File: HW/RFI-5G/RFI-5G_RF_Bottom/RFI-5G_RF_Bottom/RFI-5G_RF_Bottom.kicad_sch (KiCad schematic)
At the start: 42 parts, among them J1 Conn_01x03, J2 Conn_01x02, J3 Conn_01x03, J4 Conn_01x10, J5 SMP, J6 Conn_01x06_Female, U1 HMC8411, U2 SIM-14+, U3 LT5537, U4 LEE2-6+, U5 LEE2-6+, U7 HMC358

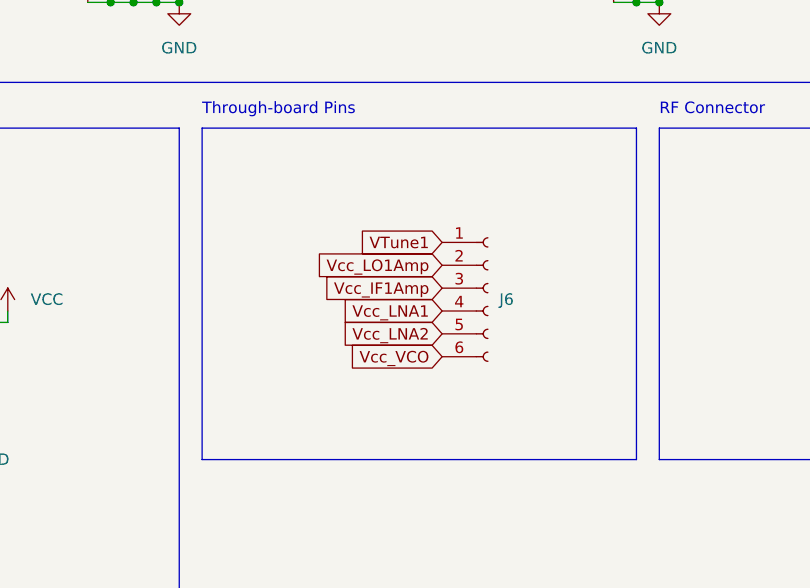
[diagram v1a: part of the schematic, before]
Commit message: PL boards
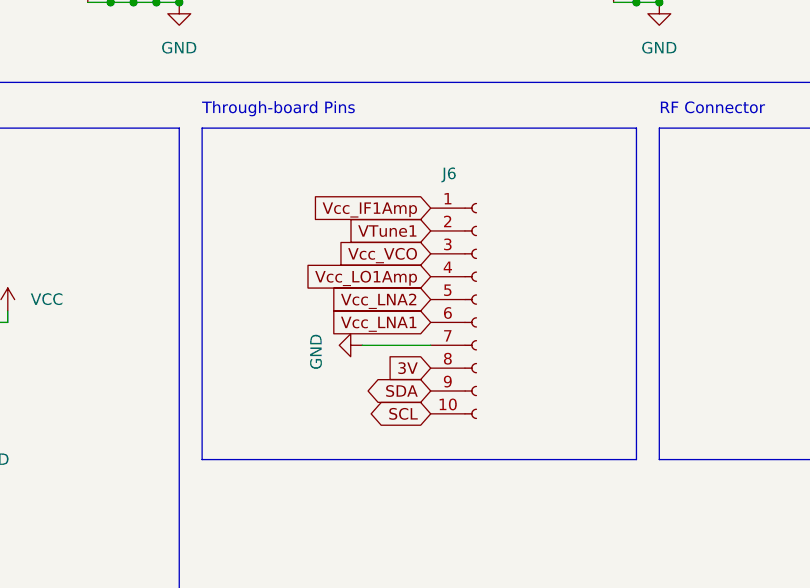
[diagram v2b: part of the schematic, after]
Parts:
- removed J6: Conn_01x06_Female, Connector_PinHeader_1.00mm:PinHeader_1x06_P1.00mm_Vertical, symbol Connector:Conn_01x06_Female
- added J6: Conn_01x10_Female, Connector_PinHeader_1.00mm:PinHeader_1x10_P1.00mm_Vertical, symbol Connector:Conn_01x10_Female
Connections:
- net 3V: now also J6.8 (Pin_8)
- net GND: now also J6.7 (Pin_7)
- net SCL: now also J6.10 (Pin_10)
- net SDA: now also J6.9 (Pin_9)
- net VTune1: now also J6.2 (Pin_2)
- net Vcc_IF1Amp: now also J6.1 (Pin_1)
- net Vcc_LNA1: now also J6.6 (Pin_6)
- net Vcc_LNA2: now also J6.5 (Pin_5)
- net Vcc_LO1Amp: now also J6.4 (Pin_4)
- net Vcc_VCO: now also J6.3 (Pin_3)
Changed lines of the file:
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@@
+    (stroke (width 0) (type default) (color 0 0 0 0))
+  )
+  (wire (pts (xy 104.14 148.59) (xy 111.76 148.59))
     (stroke (width 0) (type default) (color 0 0 0 0))
   )
@@
     (effects (font (size 1.27 1.27)) (justify left bottom))
   )
-  (global_label "Vcc_LO1Amp" (shape input) (at 113.03 139.7 180) (fields_autoplaced)
-    (effects (font (size 1.27 1.27)) (justify right))
-    (property "Intersheet References" "${INTERSHEET_REFS}" (id 0) (at 98.8845 139.6206 0)
+  (global_label "3V" (shape input) (at 111.76 151.13 180) (fields_autoplaced)
+    (effects (font (size 1.27 1.27)) (justify right))
+    (property "Intersheet References" "${INTERSHEET_REFS}" (id 0) (at 107.0488 151.0506 0)
       (effects (font (size 1.27 1.27)) (justify right) hide)
     )
@@
     )
   )
-  (global_label "Vcc_IF1Amp" (shape input) (at 113.03 142.24 180) (fields_autoplaced)
-    (effects (font (size 1.27 1.27)) (justify right))
-    (property "Intersheet References" "${INTERSHEET_REFS}" (id 0) (at 99.5498 142.1606 0)
-      (effects (font (size 1.27 1.27)) (justify right) hide)
-    )
-  )
-  (global_label "Vcc_VCO" (shape input) (at 113.03 149.86 180) (fields_autoplaced)
-    (effects (font (size 1.27 1.27)) (justify right))
-    (property "Intersheet References" "${INTERSHEET_REFS}" (id 0) (at 102.6945 149.7806 0)
-      (effects (font (size 1.27 1.27)) (justify right) hide)
-    )
-  )
   (global_label "IF1_In" (shape input) (at 76.2 39.37 180) (fields_autoplaced)
     (effects (font (size 1.27 1.27)) (justify right))
@@
     )
   )
-  (global_label "Vcc_LNA1" (shape input) (at 113.03 144.78 180) (fields_autoplaced)
-    (effects (font (size 1.27 1.27)) (justify right))
-    (property "Intersheet References" "${INTERSHEET_REFS}" (id 0) (at 101.7269 144.7006 0)
-      (effects (font (size 1.27 1.27)) (justify right) hide)
-    )
-  )
   (global_label "PoL" (shape input) (at 49.53 176.53 90) (fields_autoplaced)
     (effects (font (size 1.27 1.27)) (justify left))
@@
     )
   )
+  (global_label "Vcc_LNA2" (shape input) (at 111.76 143.51 180) (fields_autoplaced)
+    (effects (font (size 1.27 1.27)) (justify right))
+    (property "Intersheet References" "${INTERSHEET_REFS}" (id 0) (at 100.4569 143.4306 0)
+      (effects (font (size 1.27 1.27)) (justify right) hide)
+    )
+  )
   (global_label "Vcc_VCO" (shape input) (at 220.98 137.16 180) (fields_autoplaced)
     (effects (font (size 1.27 1.27)) (justify right))
@@
     )
   )
+  (global_label "Vcc_LNA1" (shape input) (at 111.76 146.05 180) (fields_autoplaced)
+    (effects (font (size 1.27 1.27)) (justify right))
+    (property "Intersheet References" "${INTERSHEET_REFS}" (id 0) (at 100.4569 145.9706 0)
+      (effects (font (size 1.27 1.27)) (justify right) hide)
+    )
+  )
   (global_label "IF1_In" (shape input) (at 165.1 139.7 180) (fields_autoplaced)
     (effects (font (size 1.27 1.27)) (justify right))
@@
     )
   )
-  (global_label "Vcc_LNA2" (shape input) (at 113.03 147.32 180) (fields_autoplaced)
-    (effects (font (size 1.27 1.27)) (justify right))
-    (property "Intersheet References" "${INTERSHEET_REFS}" (id 0) (at 101.7269 147.2406 0)
-      (effects (font (size 1.27 1.27)) (justify right) hide)
-    )
-  )
   (global_label "SDA" (shape bidirectional) (at 39.37 139.7 270) (fields_autoplaced)
     (effects (font (size 1.27 1.27)) (justify right))
@@
     )
   )
+  (global_label "VTune1" (shape input) (at 111.76 135.89 180) (fields_autoplaced)
+    (effects (font (size 1.27 1.27)) (justify right))
+    (property "Intersheet References" "${INTERSHEET_REFS}" (id 0) (at 102.6945 135.8106 0)
+      (effects (font (size 1.27 1.27)) (justify right) hide)
+    )
+  )
   (global_label "Vcc_IF2Amp2" (shape input) (at 156.21 77.47 180) (fields_autoplaced)
     (effects (font (size 1.27 1.27)) (justify right))
     (property "Intersheet References" "${INTERSHEET_REFS}" (id 0) (at 141.5202 77.3906 0)
+      (effects (font (size 1.27 1.27)) (justify right) hide)
+    )
+  )
+  (global_label "SCL" (shape bidirectional) (at 111.76 156.21 180) (fields_autoplaced)
+    (effects (font (size 1.27 1.27)) (justify right))
+    (property "Intersheet References" "${INTERSHEET_REFS}" (id 0) (at 105.8393 156.1306 0)
       (effects (font (size 1.27 1.27)) (justify right) hide)
     )
@@
     )
   )
+  (global_label "Vcc_LO1Amp" (shape input) (at 111.76 140.97 180) (fields_autoplaced)
+    (effects (font (size 1.27 1.27)) (justify right))
+    (property "Intersheet References" "${INTERSHEET_REFS}" (id 0) (at 97.6145 140.8906 0)
+      (effects (font (size 1.27 1.27)) (justify right) hide)
+    )
+  )
+  (global_label "Vcc_VCO" (shape input) (at 111.76 138.43 180) (fields_autoplaced)
+    (effects (font (size 1.27 1.27)) (justify right))
+    (property "Intersheet References" "${INTERSHEET_REFS}" (id 0) (at 101.4245 138.3506 0)
+      (effects (font (size 1.27 1.27)) (justify right) hide)
+    )
+  )
   (global_label "LO2" (shape input) (at 30.48 116.84 180) (fields_autoplaced)
     (effects (font (size 1.27 1.27)) (justify right))
@@
     )
   )
-  (global_label "VTune1" (shape input) (at 113.03 137.16 180) (fields_autoplaced)
-    (effects (font (size 1.27 1.27)) (justify right))
-    (property "Intersheet References" "${INTERSHEET_REFS}" (id 0) (at 103.9645 137.0806 0)
+  (global_label "SDA" (shape bidirectional) (at 111.76 153.67 180) (fields_autoplaced)
+    (effects (font (size 1.27 1.27)) (justify right))
+    (property "Intersheet References" "${INTERSHEET_REFS}" (id 0) (at 105.7788 153.5906 0)
       (effects (font (size 1.27 1.27)) (justify right) hide)
     )
@@
     (effects (font (size 1.27 1.27)) (justify right))
     (property "Intersheet References" "${INTERSHEET_REFS}" (id 0) (at 48.8102 77.3906 0)
+      (effects (font (size 1.27 1.27)) (justify right) hide)
+    )
+  )
+  (global_label "Vcc_IF1Amp" (shape input) (at 111.76 133.35 180) (fields_autoplaced)
+    (effects (font (size 1.27 1.27)) (justify right))
+    (property "Intersheet References" "${INTERSHEET_REFS}" (id 0) (at 98.2798 133.2706 0)
       (effects (font (size 1.27 1.27)) (justify right) hide)
     )
@@
     )
     (property "Datasheet" "" (id 3) (at 137.16 110.49 0)
+      (effects (font (size 1.27 1.27)) hide)
+    )
+    (pin "1")
+  )
+  (symbol (lib_id "power:GND") (at 104.14 148.59 270) (unit 1)
+    (in_bom yes) (on_board yes)
+    (property "Reference" "#PWR0107" (id 0) (at 97.79 148.59 0)
+      (effects (font (size 1.27 1.27)) hide)
+    )
+    (property "Value" "GND" (id 1) (at 99.06 147.32 0)
+      (effects (font (size 1.27 1.27)) (justify left))
+    )
+    (property "Footprint" "" (id 2) (at 104.14 148.59 0)
+      (effects (font (size 1.27 1.27)) hide)
+    )
+    (property "Datasheet" "" (id 3) (at 104.14 148.59 0)
       (effects (font (size 1.27 1.27)) hide)
     )
@@
     (pin "1")
   )
-  (symbol (lib_id "Connector:Conn_01x06_Female") (at 118.11 142.24 0) (unit 1)
-    (in_bom yes) (on_board yes) (fields_autoplaced)
-    (property "Reference" "J6" (id 0) (at 119.38 143.5099 0)
-      (effects (font (size 1.27 1.27)) (justify left))
-    )
-    (property "Value" "Conn_01x06_Female" (id 1) (at 119.38 144.7799 0)
-      (effects (font (size 1.27 1.27)) (justify left) hide)
-    )
-    (property "Footprint" "Connector_PinHeader_1.00mm:PinHeader_1x06_P1.00mm_Vertical" (id 2) (at 118.11 142.24 0)
-      (effects (font (size 1.27 1.27)) hide)
-    )
-    (property "Datasheet" "~" (id 3) (at 118.11 142.24 0)
-      (effects (font (size 1.27 1.27)) hide)
-    )
-    (pin "1")
-    (pin "2")
-    (pin "3")
-    (pin "4")
-    (pin "5")
-    (pin "6")
-  )
   (symbol (lib_id "power:GND") (at 222.25 85.09 0) (unit 1)
     (in_bom yes) (on_board yes) (fields_autoplaced)
@@
     (pin "1")
   )
+  (symbol (lib_id "Connector:Conn_01x10_Female") (at 116.84 143.51 0) (unit 1)
+    (in_bom yes) (on_board yes)
+    (property "Reference" "J6" (id 0) (at 113.03 129.54 0)
+      (effects (font (size 1.27 1.27)) (justify left))
+    )
+    (property "Value" "Conn_01x10_Female" (id 1) (at 118.11 146.0499 0)
+      (effects (font (size 1.27 1.27)) (justify left) hide)
+    )
+    (property "Footprint" "Connector_PinHeader_1.00mm:PinHeader_1x10_P1.00mm_Vertical" (id 2) (at 116.84 143.51 0)
+      (effects (font (size 1.27 1.27)) hide)
+    )
+    (property "Datasheet" "~" (id 3) (at 116.84 143.51 0)
+      (effects (font (size 1.27 1.27)) hide)
+    )
+    (pin "1")
+    (pin "10")
+    (pin "2")
+    (pin "3")
+    (pin "4")
+    (pin "5")
+    (pin "6")
+    (pin "7")
+    (pin "8")
+    (pin "9")
+  )
   (symbol (lib_id "power:GND") (at 59.69 144.78 0) (unit 1)
     (in_bom yes) (on_board yes) (fields_autoplaced)
@@
       (reference "#PWR0106") (unit 1) (value "GND") (footprint "")
     )
+    (path "/35519fd5-08ff-4fab-91c9-037e2a0c1c90"
+      (reference "#PWR0107") (unit 1) (value "GND") (footprint "")
+    )
     (path "/28b84f01-4b1c-4220-bcbc-a91fb9c17242"
       (reference "C1") (unit 1) (value "100nF") (footprint "Capacitor_SMD:C_0402_1005Metric")
@@
       (reference "J5") (unit 1) (value "SMP") (footprint "GGS_Connectors:SMP_StraightPlugPCB")
     )
-    (path "/bfa21043-576f-49ac-8f69-17c49a0821d4"
-      (reference "J6") (unit 1) (value "Conn_01x06_Female") (footprint "Connector_PinHeader_1.00mm:PinHeader_1x06_P1.00mm_Vertical")
+    (path "/f55b2315-ffcf-45cb-b8d5-dd0439b81933"
+      (reference "J6") (unit 1) (value "Conn_01x10_Female") (footprint "Connector_PinHeader_1.00mm:PinHeader_1x10_P1.00mm_Vertical")
     )
     (path "/6ba90c57-8775-4815-9ae3-5af56b73607e"
